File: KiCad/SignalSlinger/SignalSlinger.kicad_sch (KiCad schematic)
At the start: 65 parts, among them J101 Conn_01x02, J103 Conn_01x02, J104 Conn_01x02, J105 Conn_01x02, J106 Conn_01x02, J107 DB9 Female, J108 Conn_01x02, J109 Conn_01x03, J110 Conn_01x02, J111 Conn_01x03, J112 External Power Source, J113 Controlled Power, P101 ISP/PDI, Q101 BSS84W-7-F, Q102 BSS138W-7-F, Q103 IRF610, SW101 SW_SPST, U101 AVR128DA28, U102 SI5351, U103 TPS22810DBVT, U104 LM5134, U105 TPS22810DBVT, X101 SIT1566AC TCO, X102 25 MHz

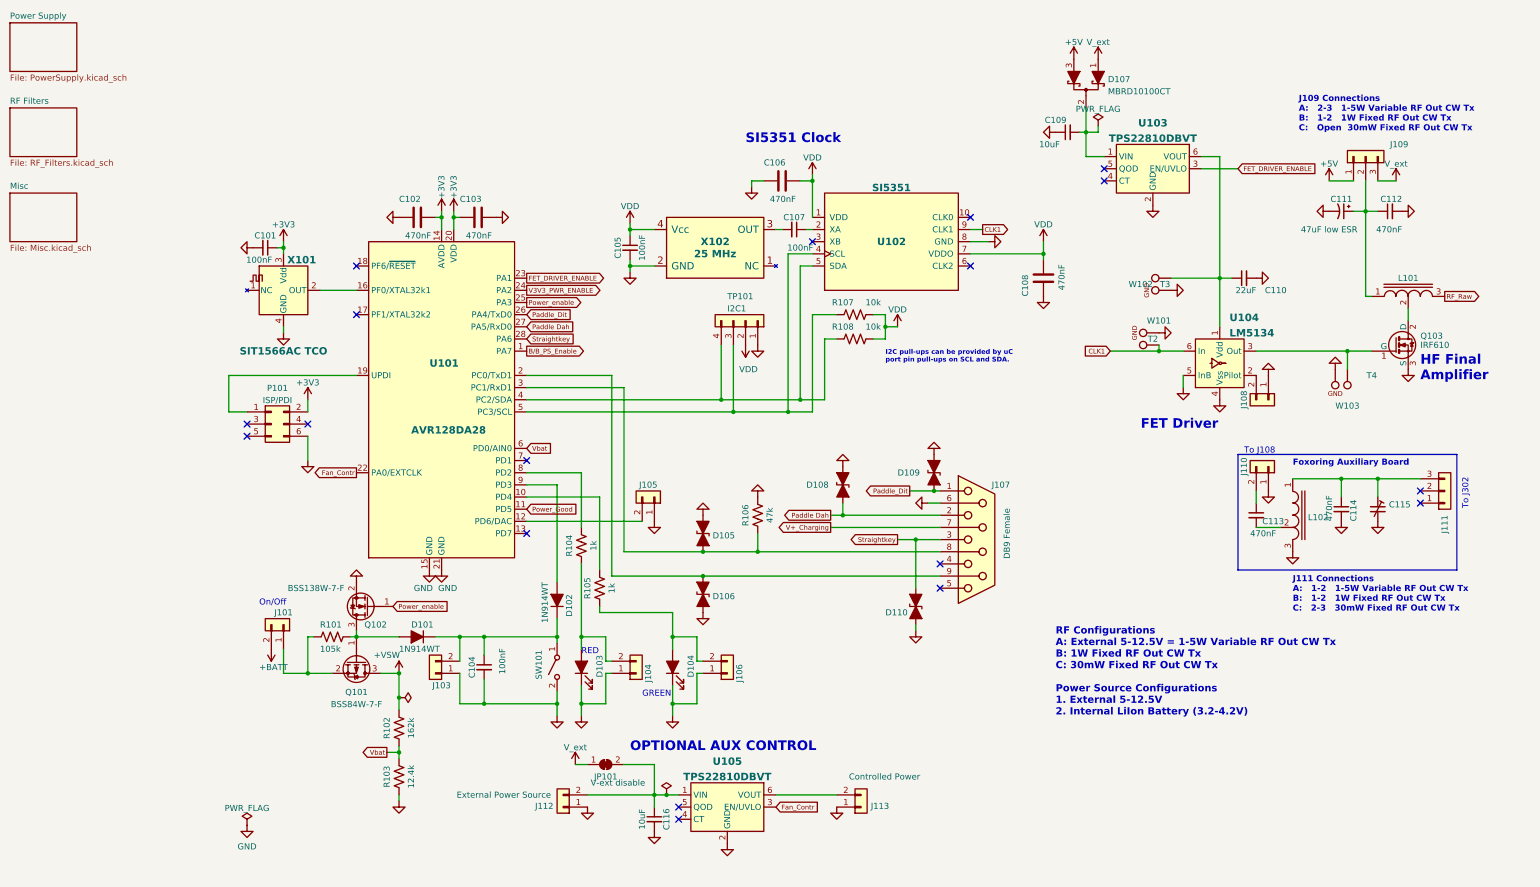
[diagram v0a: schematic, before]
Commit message: Updates
o Updated Gerbers
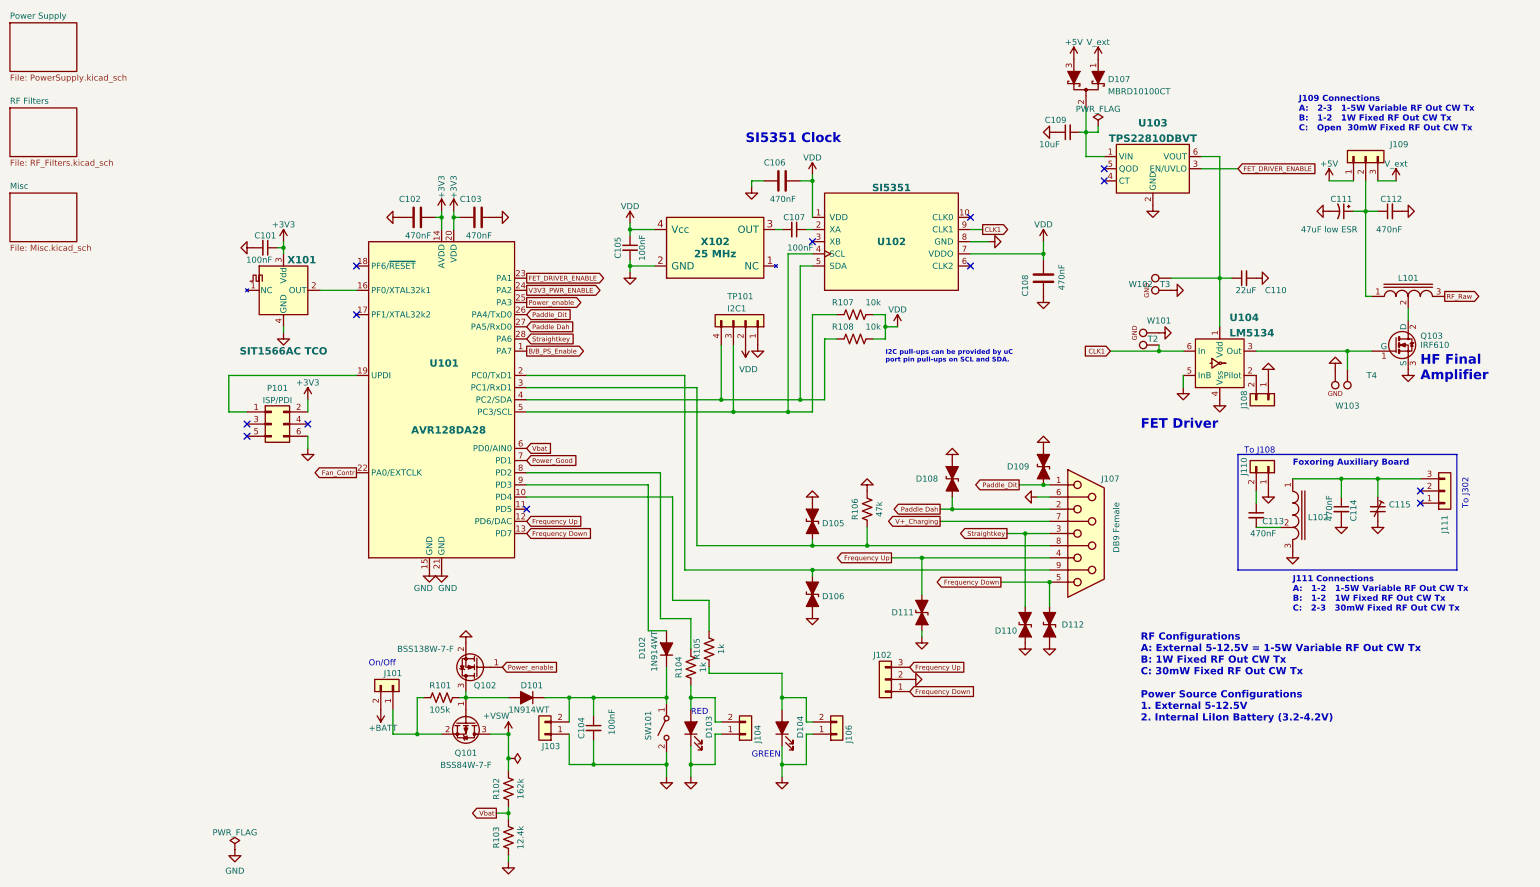
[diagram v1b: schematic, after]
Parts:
- removed C116: 10uF, Capacitor_SMD:C_0805_2012Metric, symbol Device:C_Small
- removed J105: Conn_01x02, Connector_PinSocket_2.54mm:PinSocket_1x02_P2.54mm_Vertical, symbol Connector_Generic:Conn_01x02
- removed J112: External Power Source, Connector_PinHeader_2.54mm:PinHeader_1x02_P2.54mm_Vertical, symbol Connector_Generic:Conn_01x02
- removed J113: Controlled Power, Connector_PinHeader_2.54mm:PinHeader_1x02_P2.54mm_Vertical, symbol Connector_Generic:Conn_01x02
- removed JP101: V-ext disable, Jumper:SolderJumper-2_P1.3mm_Bridged_RoundedPad1.0x1.5mm, symbol Jumper:SolderJumper_2_Bridged
- removed U105: TPS22810DBVT, Package_TO_SOT_SMD:SOT-23-6, symbol Power_Management:TPS22810DBVT
- added D111, D112: ESD9B5.0ST5G_1, Diode_SMD:D_0603_1608Metric, symbol Diode:ESD9B5.0ST5G_1
- added J102: Conn_01x03, Connector_PinHeader_2.54mm:PinHeader_1x03_P2.54mm_Vertical, symbol Connector_Generic:Conn_01x03
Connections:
- net GND: now also D111.2 (A2), D112.2 (A2), J102.2 (Pin_2)
- net Power_Good: now also U101.7 (PD1); no longer U101.11 (PD5)
- net Frequency Up: now reaches U101.12 (PD6/DAC)
- net Frequency Up: now also J107.4, D111.1 (A1), J102.3 (Pin_3)
- net Frequency Down: now reaches U101.13 (PD7)
- net Frequency Down: now also J107.5, D112.1 (A1), J102.1 (Pin_1)
- no-connect marks 18 -> 13
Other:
- note removed: "OPTIONAL AUX CONTROL"
- moved on the sheet: C104, D101, D102, D103, D104, D105, D106, D108, D109, D110, J101, J103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
